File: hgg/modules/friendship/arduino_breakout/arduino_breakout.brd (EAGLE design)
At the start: 105.6 x 67.3 mm, 23 parts, among them IC1 MAX481CSA, IC2 MAX481CSA, IC3 74AC165D, IC4 4517, IC5 74AC165D, IC6 74AC165D, IC7 74AC393D, IC8 74AC393D, IC9 74AC393D

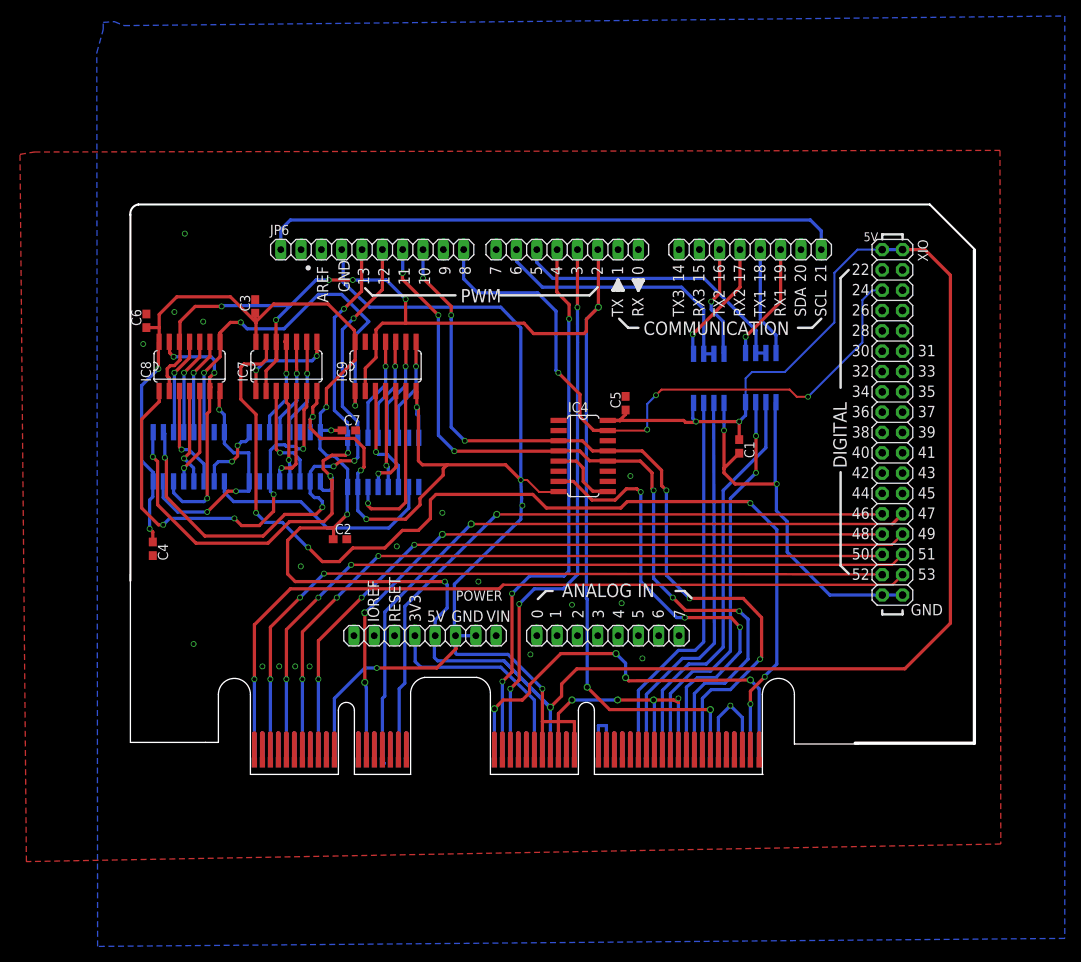
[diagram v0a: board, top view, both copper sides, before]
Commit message: small routing improvements
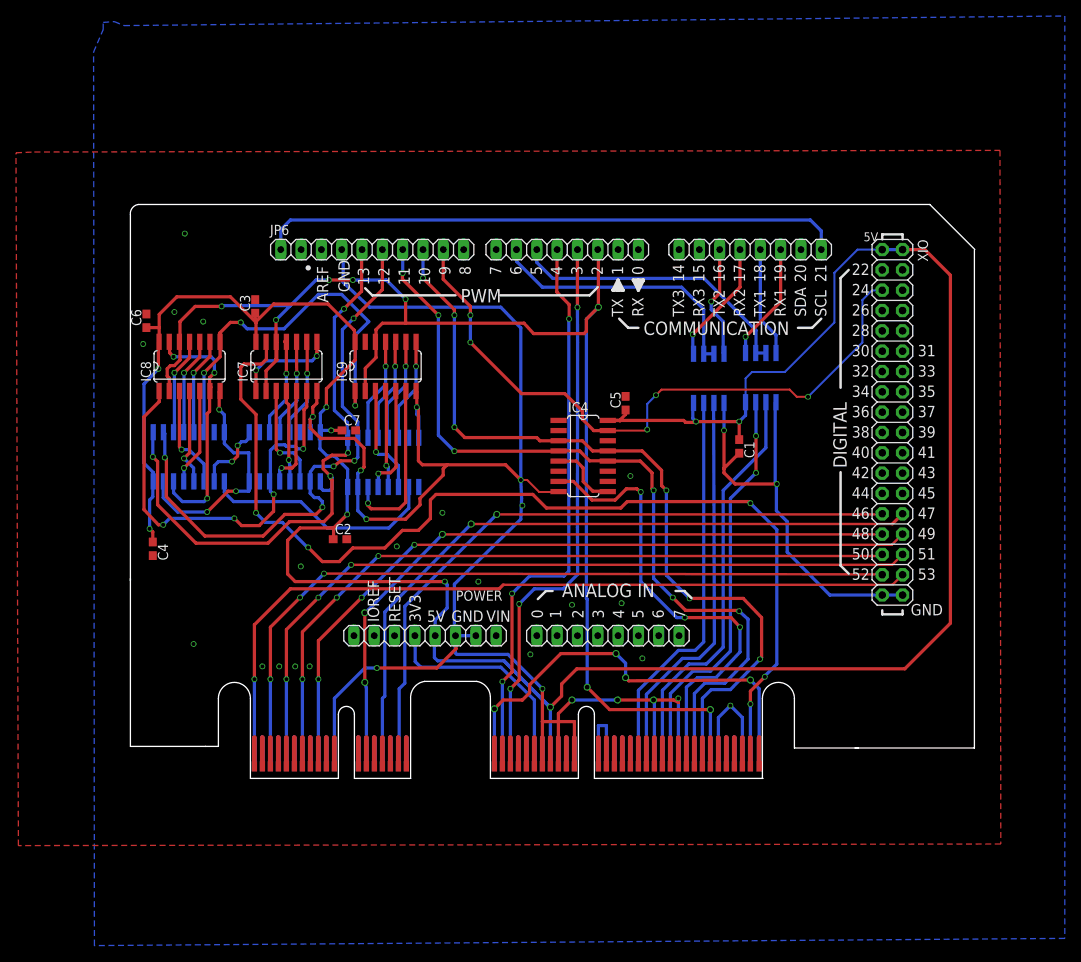
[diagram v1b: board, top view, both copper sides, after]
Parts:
- moved U$1 0.50 mm to (-0.90, 17.1)
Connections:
- removed net PH6: JP6.9
- new net PH5: JP6.10
- net SLOWTIMESER: now also JP6.9; no longer JP6.10
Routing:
- net GND: track 342.2 -> 346.2 mm
- net PRESENT: track 55.4 -> 56.4 mm
- net N$1: track 10.2 -> 11.2 mm
- net SLOWCLKMOSI: track 59.0 -> 59.5 mm
- net SLOWCLKCLK: track 103.1 -> 103.6 mm
- net PRSNTDATAIN: track 97.5 -> 98.0 mm
- net PPS: track 176.3 -> 176.8 mm
- net N$6: track 51.7 -> 52.2 mm
- net N$5: track 50.8 -> 51.3 mm
- net N$3: track 49.7 -> 50.2 mm
- net N$2: track 49.5 -> 50.0 mm
- net IRQDATAIN: track 100.8 -> 101.3 mm
- net IRQ: track 96.2 -> 96.7 mm
- net INTACKSER: track 87.5 -> 88.0 mm
- net INTACKSCK: track 92.8 -> 93.3 mm
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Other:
- board size 105.6 x 67.3 mm -> 105.6 x 67.9 mm
